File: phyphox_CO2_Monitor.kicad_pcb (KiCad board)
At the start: 2 copper layers, 80 x 38 mm, 10 parts

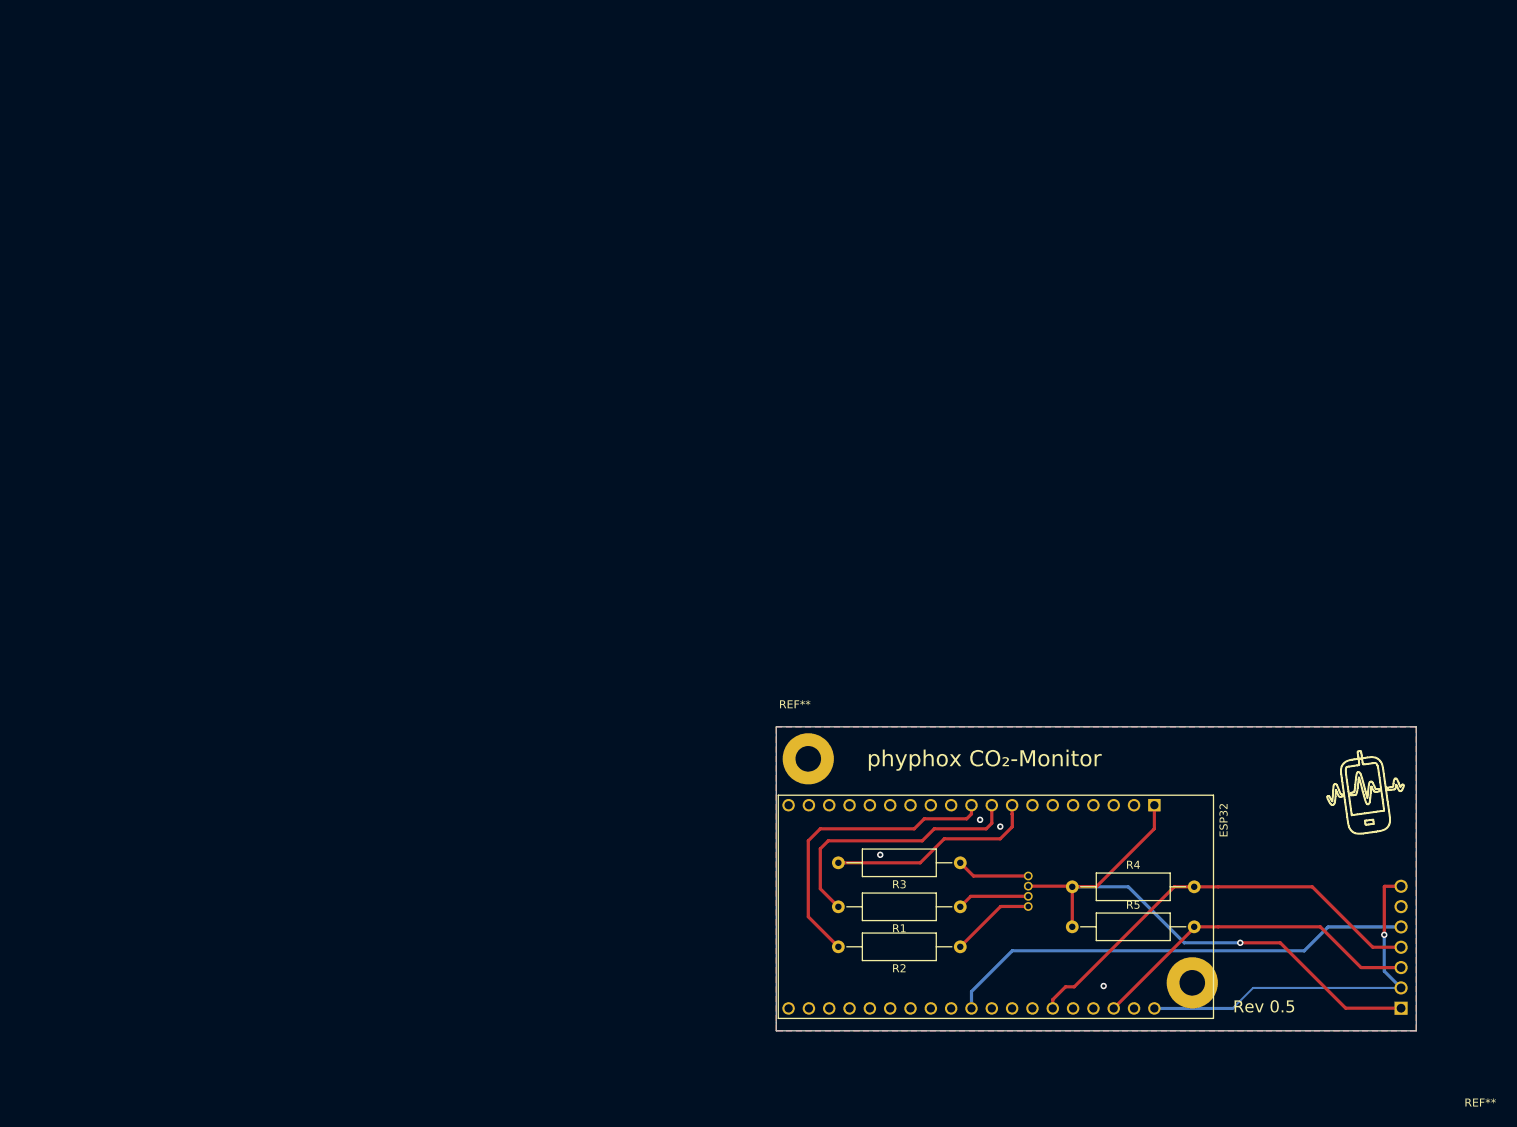
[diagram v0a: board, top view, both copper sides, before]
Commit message: horizontal design
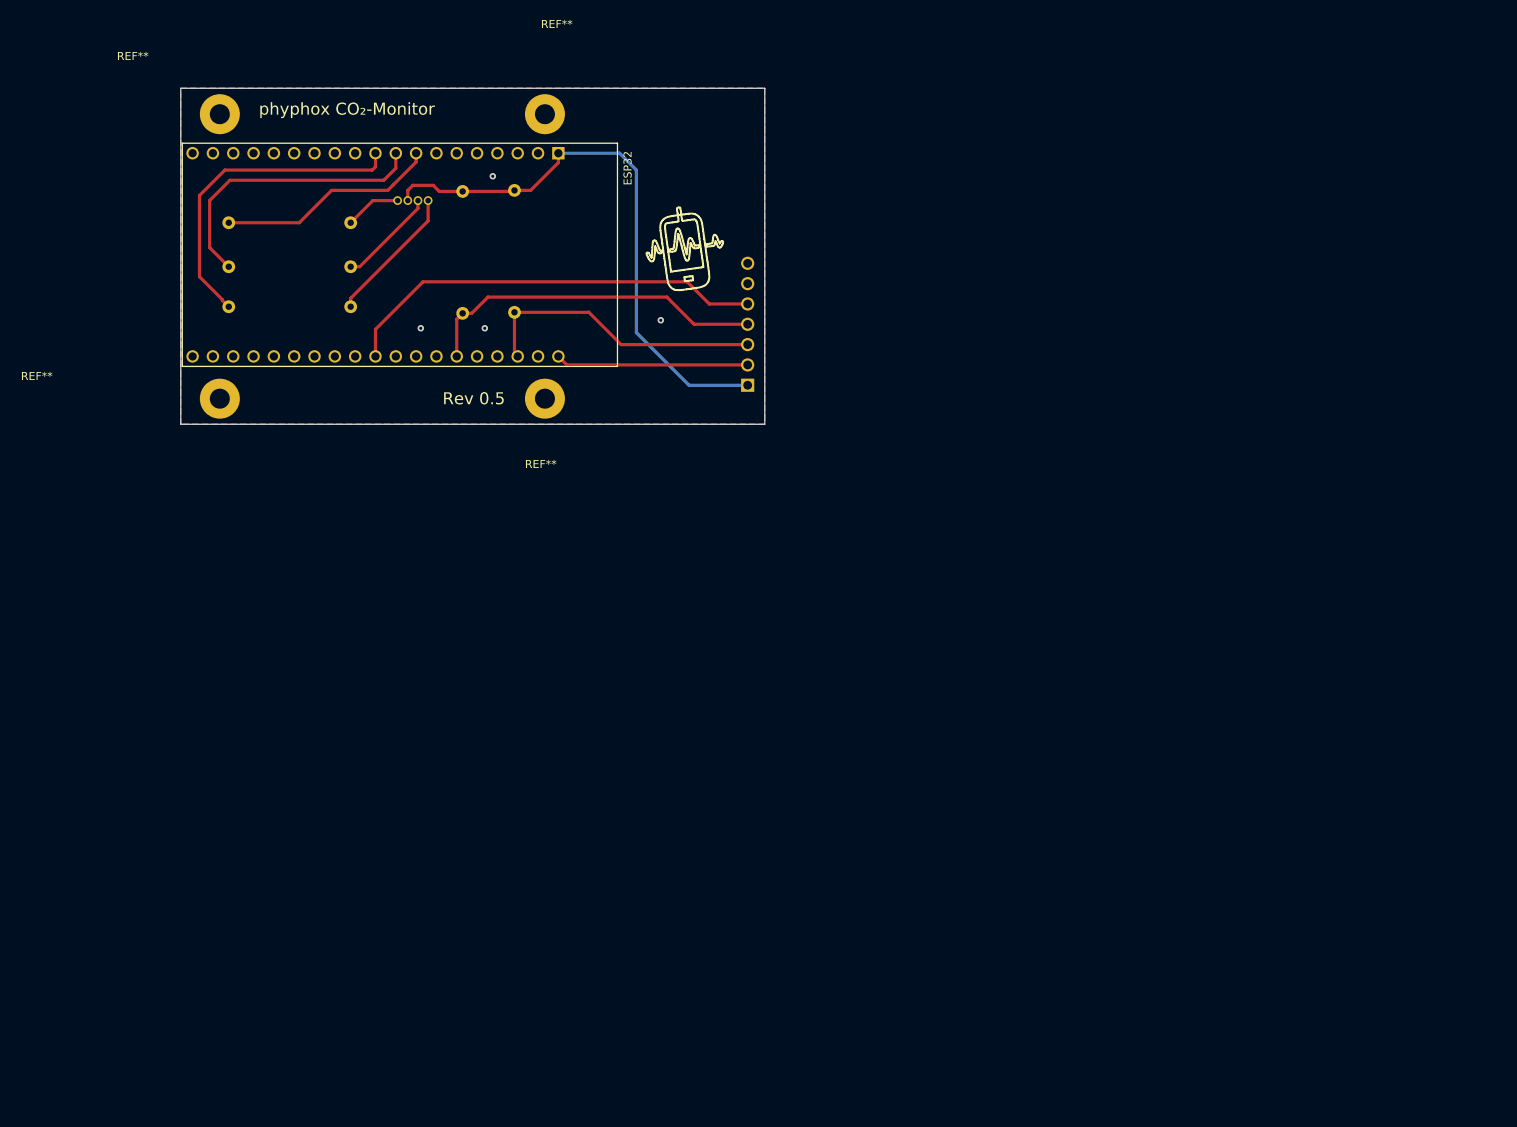
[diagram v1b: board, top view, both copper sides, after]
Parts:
- removed the REF** at (51.0, 63.0)
- removed the REF** at (99.0, 91.0)
- added REF**: MountingHole_2.5mm_Pad, MountingHole:MountingHole_2.5mm_Pad, F.Cu at (18.1, 18.0)
- added REF**: MountingHole_2.5mm_Pad, MountingHole:MountingHole_2.5mm_Pad, F.Cu at (18.1, -17.6)
- added REF**: MountingHole_2.5mm_Pad, MountingHole:MountingHole_2.5mm_Pad, F.Cu at (-22.6, -17.6)
- added REF**: MountingHole_2.5mm_Pad, MountingHole:MountingHole_2.5mm_Pad, F.Cu at (-22.6, 18.0)
- R1, R2, R3, R4, R5: moved to B.Cu
- moved RGB-LED 116.2 mm to (6.02, -6.78), turned to 270 degrees
- moved R4 115.6 mm to (7.80, -7.92), turned to 270 degrees
- moved R5 115.5 mm to (14.3, -8.05), turned to 270 degrees
- moved SCD30 112.8 mm to (33.3, 0.20)
- moved R1 110.5 mm to (-6.20, 1.49)
- moved R2 110.5 mm to (-6.20, 6.49)
- moved R3 110.5 mm to (-6.20, -4.01)
- moved ESP32 110.4 mm to (0.00, 0.00)
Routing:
- net GND: track 47.5 -> 24.1 mm, vias 5 -> 4
- net SDA: track 53.6 -> 43.6 mm
- net Net-(D1-Pad4): track 10.6 -> 17.3 mm
- net SCL: track 42.3 -> 36.5 mm
- net RDY: track 59.1 -> 53.5 mm
- net Net-(D1-Pad3): track 9.04 -> 12.4 mm
- net VDD: track 74.1 -> 71.0 mm, vias 1 -> 0
- net GREEN: track 37.7 -> 40.6 mm
- net RED: track 33.2 -> 36.1 mm
- net Net-(D1-Pad1): track 9.18 -> 7.02 mm
- net BLUE: track 26.3 -> 27.7 mm
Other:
- board size 80 x 38 mm -> 73 x 42 mm
